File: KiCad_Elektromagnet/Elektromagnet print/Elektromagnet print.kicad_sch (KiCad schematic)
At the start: 5 parts

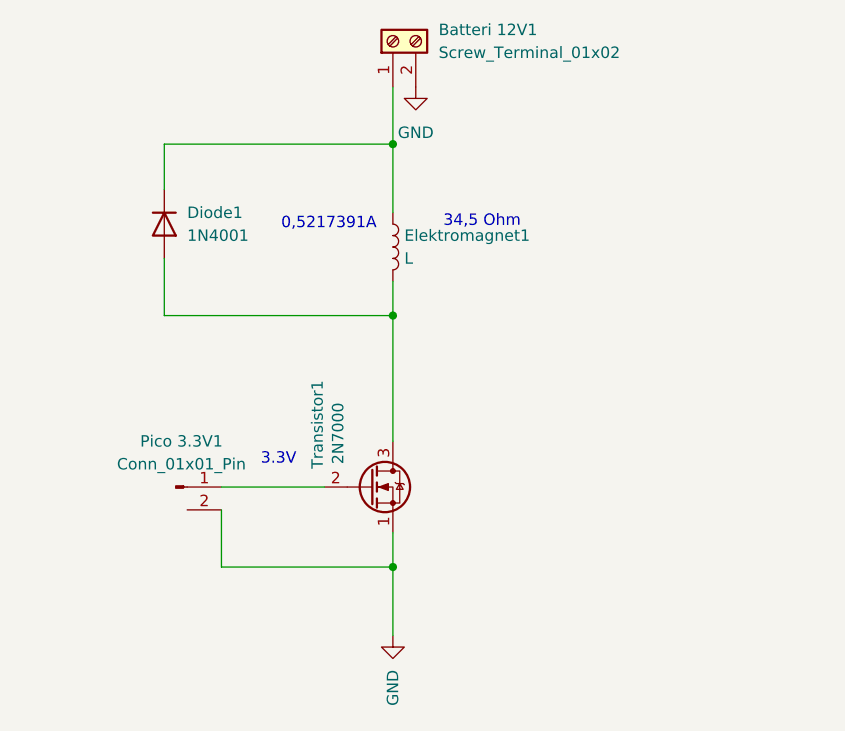
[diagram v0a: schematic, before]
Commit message: Bare haft kigget på KiCad tegningerne
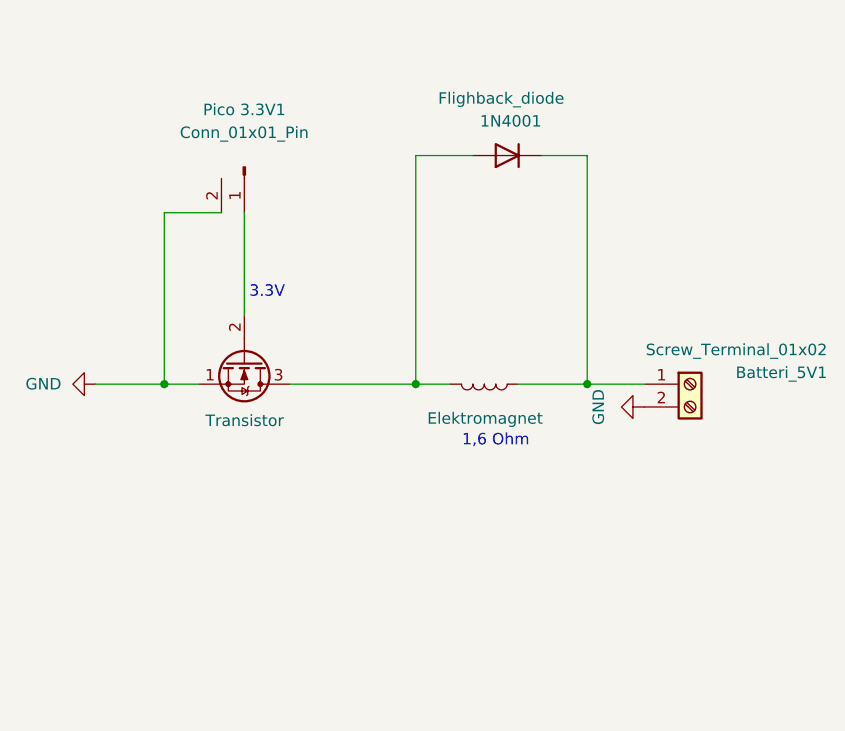
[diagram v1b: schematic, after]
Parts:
- Batteri_5V1: renamed from Batteri 12V1
- renumbered Elektromagnet1 to Elektromagnet, Diode1 to Flighback_diode, Transistor1 to Transistor
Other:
- note added: "1,6 Ohm"
- note removed: "0,5217391A"
- note removed: "34,5 Ohm"
- moved on the sheet: Batteri_5V1, Elektromagnet, Flighback_diode, Pico 3.3V1, Transistor
